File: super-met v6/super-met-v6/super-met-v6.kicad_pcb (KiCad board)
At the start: 4 copper layers, 75.1 x 95.1 mm, 68 parts, among them J1 Conn_01x02, J2 Conn_01x08, J3 Conn_01x08, J4 Conn_01x04, J5 Conn_01x08, J6 Conn_01x04, J7 Conn_01x02, J8 Conn_01x02, Q1 AO3400A, Q10 AO3400A, Q11 AO3400A, Q12 AO3400A, Q2 AO3400A, Q3 AO3400A, Q4 AO3400A, Q5 AO3400A, Q6 AO3400A, Q7 AO3400A, Q8 AO3400A, Q9 AO3400A, U1 DC-DC_MOD, U10 74HC595, U11 GY-GPS6MV2, U12 ESP-01v090, U13 74HC4052D, U14 BLUEPILL, U2 DC-DC_MOD, U3 DC-DC_MOD, U4 ADS1115IDGS, U5 ADS1115IDGS, U6 ADS1115IDGS, U7 ADS1115IDGS, U8 74HC595, U9 SIM800L

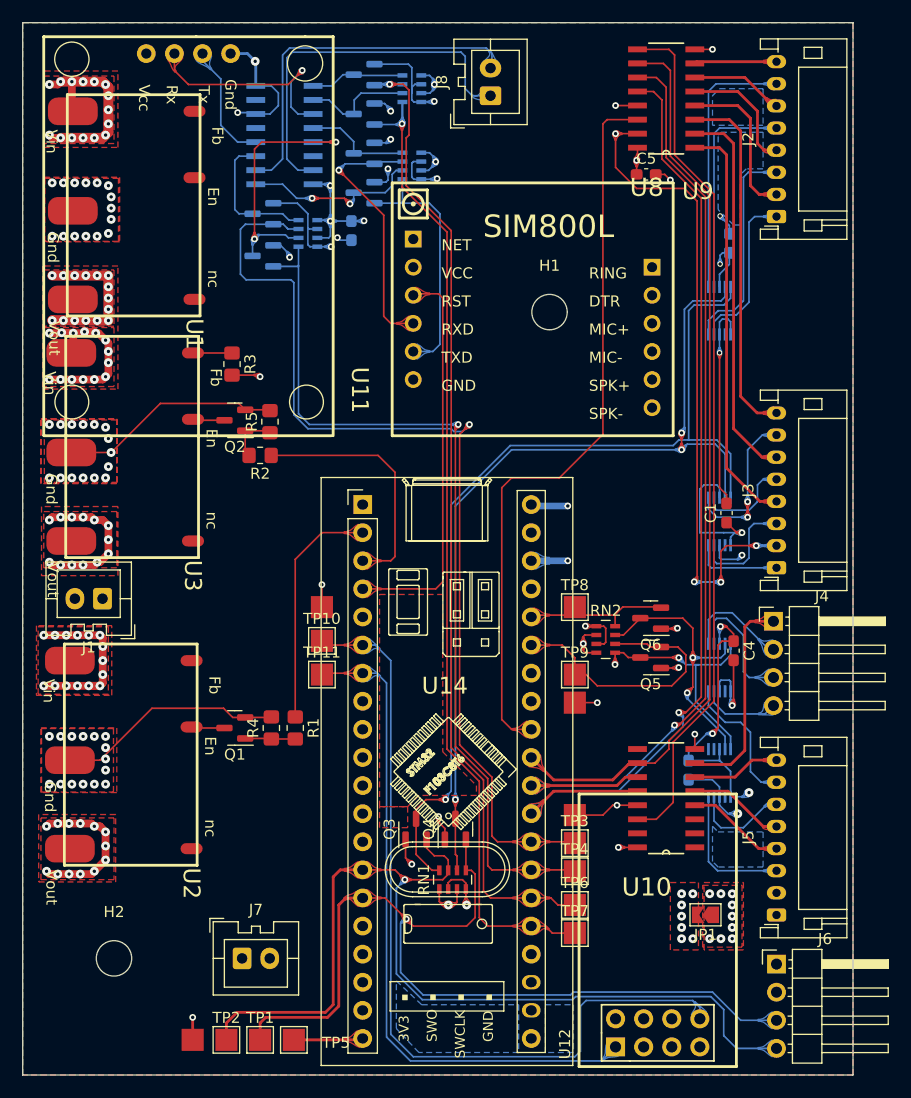
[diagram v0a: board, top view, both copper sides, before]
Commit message: almost done ?
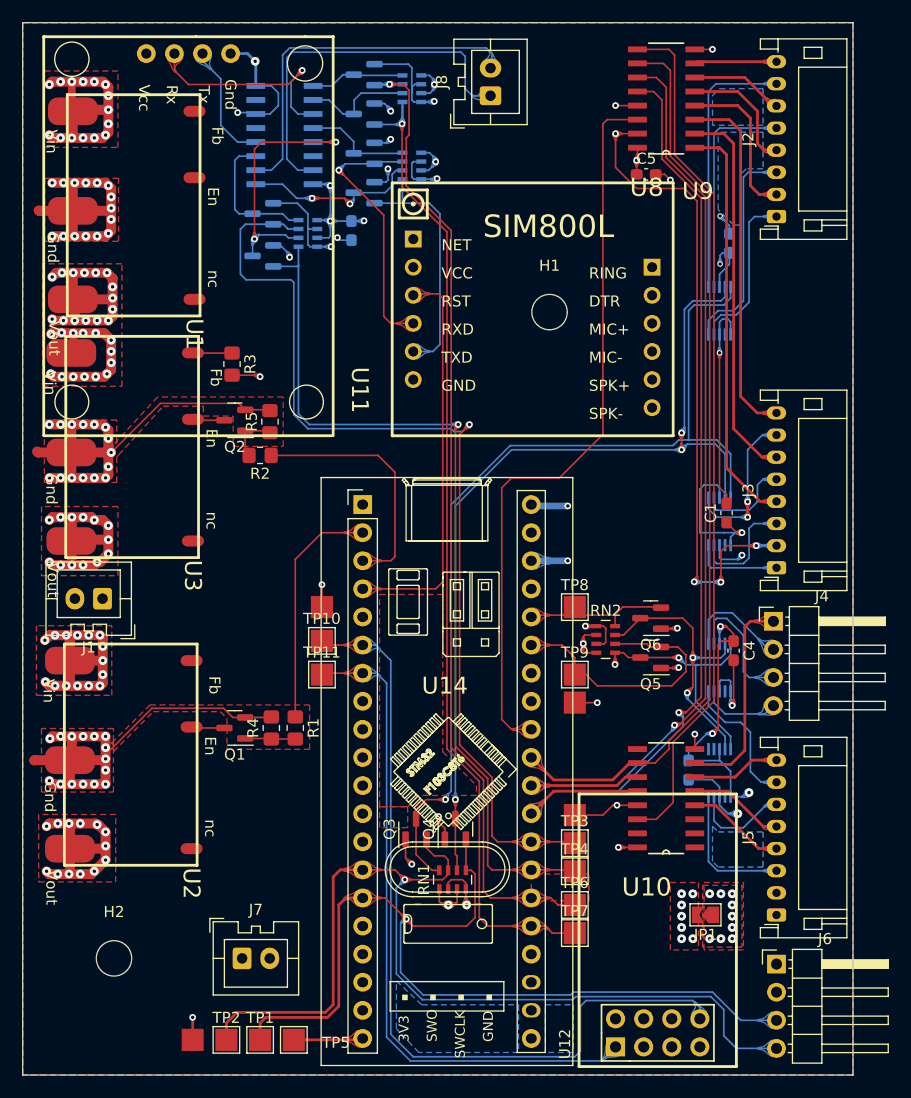
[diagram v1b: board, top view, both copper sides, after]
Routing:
- net GND: track 76.2 -> 155.2 mm
- net /Power_Vin: track 50.1 -> 73.5 mm
- net 3.3v: track 119.9 -> 128.2 mm
- net 5.2v: track 323.6 -> 331.6 mm
- net 4.2v: track 55.1 -> 62.9 mm
- removed copper zone on F.Cu, net /Power_Vin
- removed copper zone on F.Cu, net 3.3v
- removed copper zone on F.Cu, net 4.2v
- removed copper zone on F.Cu, net 5.2v
